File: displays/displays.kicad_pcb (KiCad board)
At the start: 2 copper layers, 59 x 52.8 mm, 105 parts, among them U10 TZ-H1010-RGB/A-BU08UF-TA1305N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, U11 TZ-H1010-RGB/A-BU08UF-TA1305N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, U12 TZ-H1010-RGB/A-BU08UF-TA1305N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, U13 TZ-H1010-RGB/A-BU08UF-TA1305N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, U14 TZ-H1010-RGB/A-BU08UF-TA1305N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, U15 TZ-H1010-RGB/A-BU08UF-TA1305N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, U16 TZ-H1010-RGB/A-BU08UF-TA1305N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, U17 TZ-H1010-RGB/A-BU08UF-TA1305N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, U18 TZ-H1010-RGB/A-BU08UF-TA1305N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, U19 TZ-H1010-RGB/A-BU08UF-TA1305N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, U2 TZ-H1010-RGB/A-BU08UF-TA1305N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, U20 TZ-H1010-RGB/A-BU08UF-TA1305N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, U21 TZ-H1010-RGB/A-BU08UF-TA1305N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, U22 TZ-H1010-RGB/A-BU08UF-TA1305N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, U23 TZ-H1010-RGB/A-BU08UF-TA1305N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, U24 TZ-H1010-RGB/A-BU08UF-TA1305N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, U25 TZ-H1010-RGB/A-BU08UF-TA1305N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, U26 TZ-H1010-RGB/A-BU08UF-TA1305N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, U27 TZ-H1010-RGB/A-BU08UF-TA1305N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, U28 TZ-H1010-RGB/A-BU08UF-TA1305N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, U29 TZ-H1010-RGB/A-BU08UF-TA1305N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, U3 TZ-H1010-RGB/A-BU08UF-TA1305N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, U30 TZ-H1010-RGB/A-BU08UF-TA1305N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, U31 TZ-H1010-RGB/A-BU08UF-TA1305N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, U32 TZ-H1010-RGB/A-BU08UF-TA1305N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, U33 TZ-H1010-RGB/A-BU08UF-TA1305N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, U34 TZ-H1010-RGB/A-BU08UF-TA1305N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, U35 TZ-H1010-RGB/A-BU08UF-TA1305N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, U36 TZ-H1010-RGB/A-BU08UF-TA1305N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, U37 TZ-H1010-RGB/A-BU08UF-TA1305N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, U38 TZ-H1010-RGB/A-BU08UF-TA1305N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, U39 TZ-H1010-RGB/A-BU08UF-TA1305N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, U4 TZ-H1010-RGB/A-BU08UF-TA1305N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, U40 TZ-H1010-RGB/A-BU08UF-TA1305N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, U41 TZ-H1010-RGB/A-BU08UF-TA1305N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, U42 TZ-H1010-RGB/A-BU08UF-TA1305N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, U43 TZ-H1010-RGB/A-BU08UF-TA1305N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, U44 PJ-320A-4P DIP, U45 TPA6132A2RTER, U46 74LVC2G17GV_C53954310, U47 74LVC2G17GV_C53954310, U48 74LVC2G17GV_C53954310, U5 TZ-H1010-RGB/A-BU08UF-TA1305N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, U6 TZ-H1010-RGB/A-BU08UF-TA1305N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, U7 TZ-H1010-RGB/A-BU08UF-TA1305N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, U8 TZ-H1010-RGB/A-BU08UF-TA1305N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, U9 TZ-H1010-RGB/A-BU08UF-TA1305N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

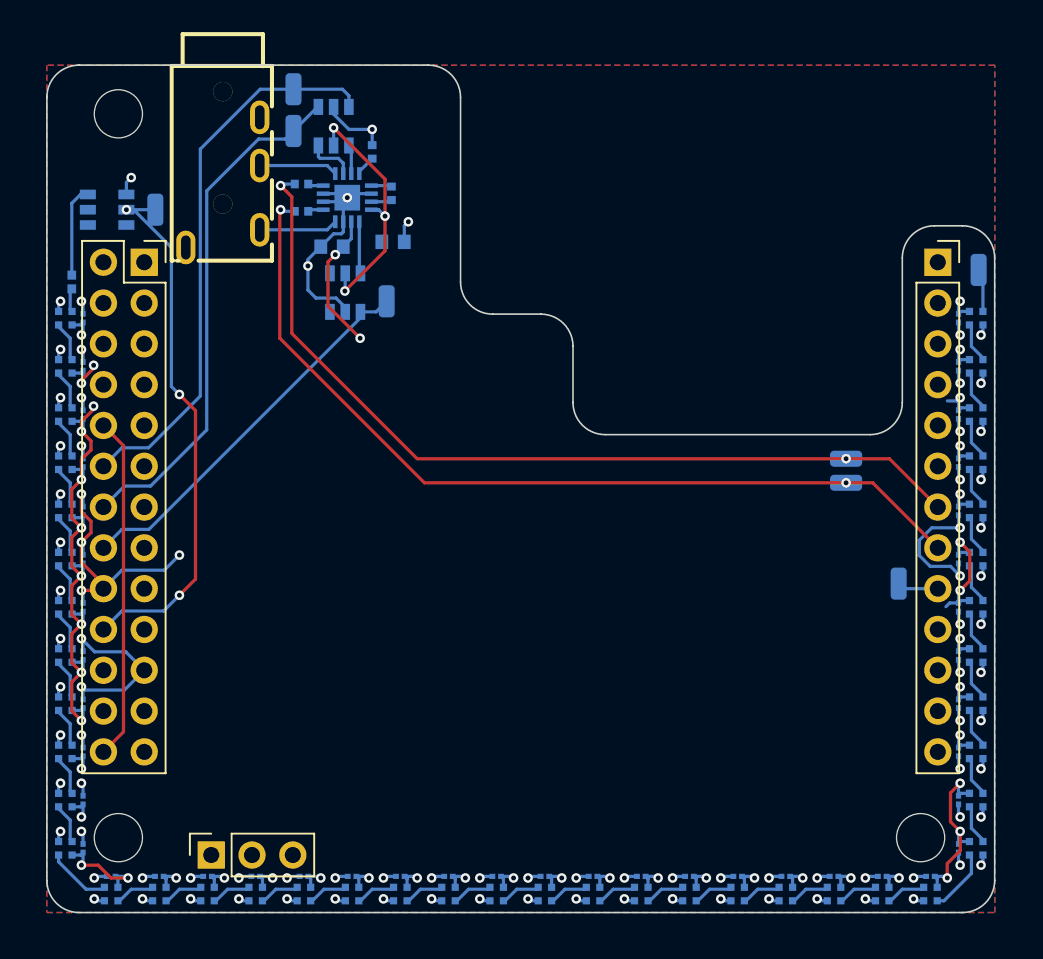
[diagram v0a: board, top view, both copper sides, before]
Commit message: updated board
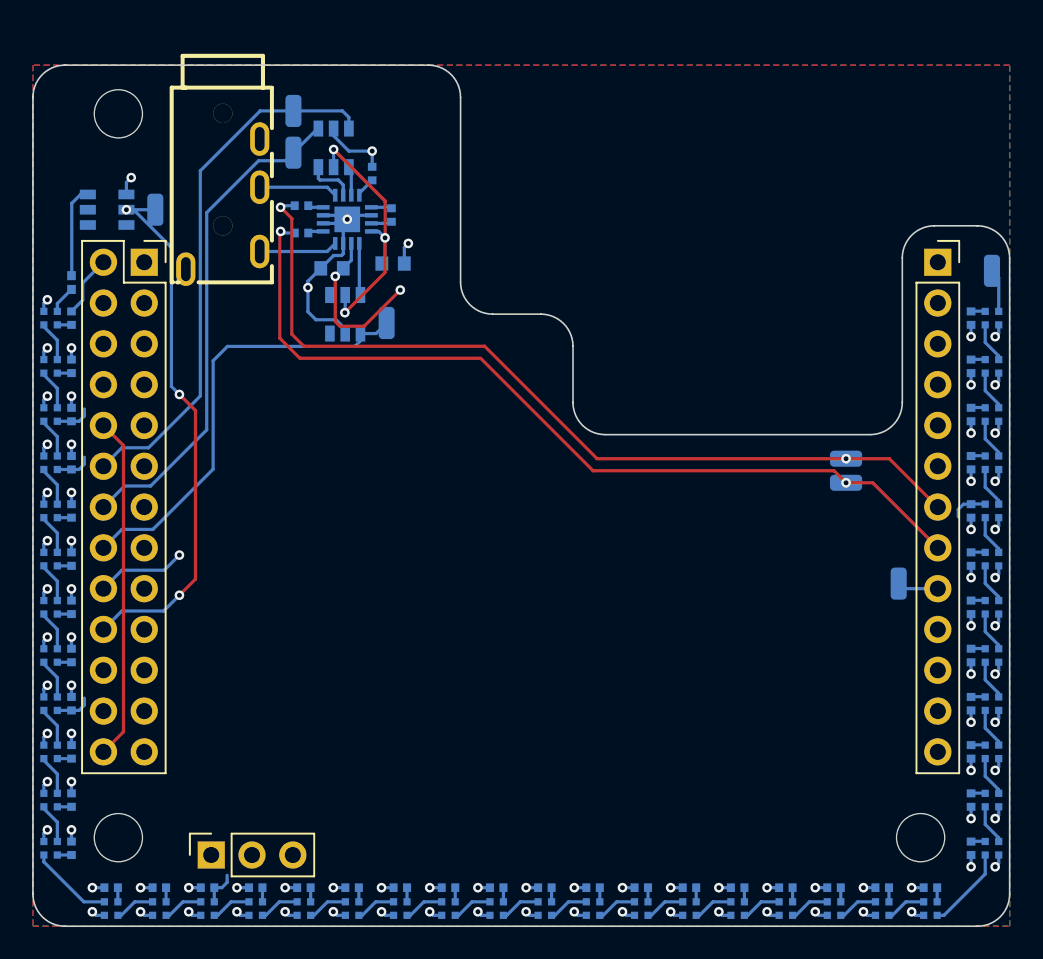
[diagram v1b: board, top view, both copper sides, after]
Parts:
- C1, C10, C11, C12, C13, C14, C15, C16, C17, C18, C19, C2, C20, C21, C22, C23, C24, C25, C26, C27, C28, C29, C3, C30, C31, C32, C33, C34, C35, C36, C37, C38, C39, C4, C40, C41, C42, C5, C6, C7, C8, C9: footprint lcsc_footprints:C307380_C0201 -> lcsc_footprints:C1525_C0402
- C43, C44, C45, C47: footprint lcsc_footprints:C29266_C0402 -> lcsc_footprints:C52923_C0402
- R1: value 500 -> 200; footprint lcsc_footprints:C6460545_R0402 -> lcsc_footprints:C25087_R0402
- moved C44 1.35 mm to (34.1, 24.8)
- moved C45 1.35 mm to (38.5, 22.8)
- moved C46 1.35 mm to (39.8, 28.4)
- moved TP6 1.35 mm to (33.6, 18.9)
- moved U45 1.35 mm to (37.0, 25.6)
- moved C43 1.35 mm to (34.1, 26.4)
- moved C47 1.35 mm to (39.7, 25.3)
- moved C48 1.35 mm to (36.0, 28.6)
- moved TP4 1.35 mm to (39.4, 32.0)
- moved TP5 1.35 mm to (33.6, 21.4)
- moved U44 1.35 mm to (29.2, 24.6)
- moved U46 1.35 mm to (36.8, 31.5)
- moved U47 1.35 mm to (36.1, 21.1)
- moved U27 0.98 mm to (77.1, 49.8)
- moved U29 0.98 mm to (77.1, 52.8)
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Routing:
- net +5V: track 113.9 -> 54.2 mm, vias 46 -> 2
- net GND: track 114.4 -> 94.9 mm, vias 90 -> 89
- net /AMPEN: track 24.2 -> 27.6 mm
- net /LINEOUTL: track 55.3 -> 54.0 mm
- net /AMPG1: track 34.9 -> 33.5 mm
- net /AMPG0: track 32.4 -> 31.1 mm
- net /LINEOUTR: track 55.1 -> 53.8 mm
- net Net-(U36-DO): track 4.03 -> 5.24 mm
- net Net-(U13-DO): track 4.03 -> 5.22 mm
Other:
- board size 59 x 52.8 mm -> 60.8 x 53.6 mm
